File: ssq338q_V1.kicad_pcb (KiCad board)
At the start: 6 copper layers, 32 x 40 mm, 126 parts, among them J4 Conn_01x04_MountingPin, J6 Conn_01x06_MountingPin, J7 Conn_01x03_MountingPin, J8 Conn_01x02_MountingPin, U1 TLV74018PDBVR, U11 W25Q128JVSIQ, U13 BL-M8812EU2, U14 TMI3411, U17 TMI3408F, U2 SSC338Q, U3 MP9943GQ-Z, U7 TMI3113B, X2 24MHz

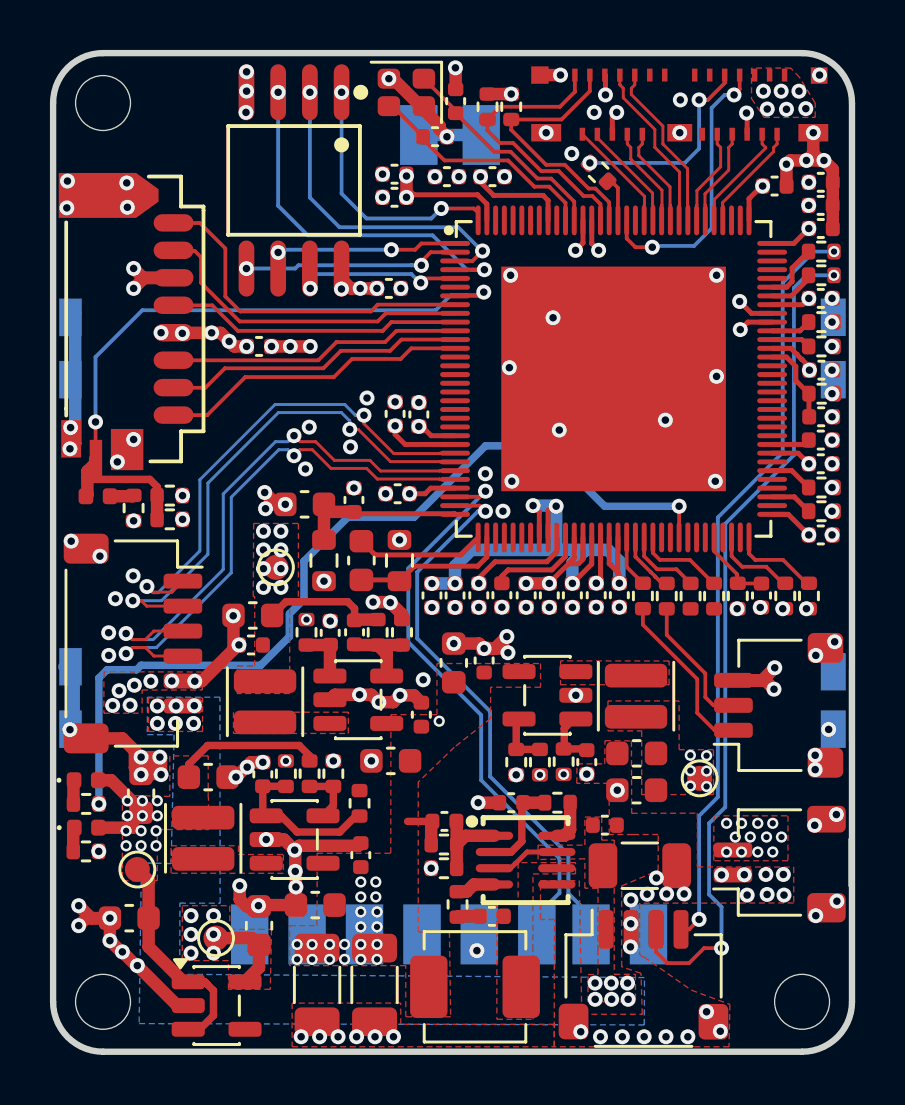
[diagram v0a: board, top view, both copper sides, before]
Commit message: minor changes
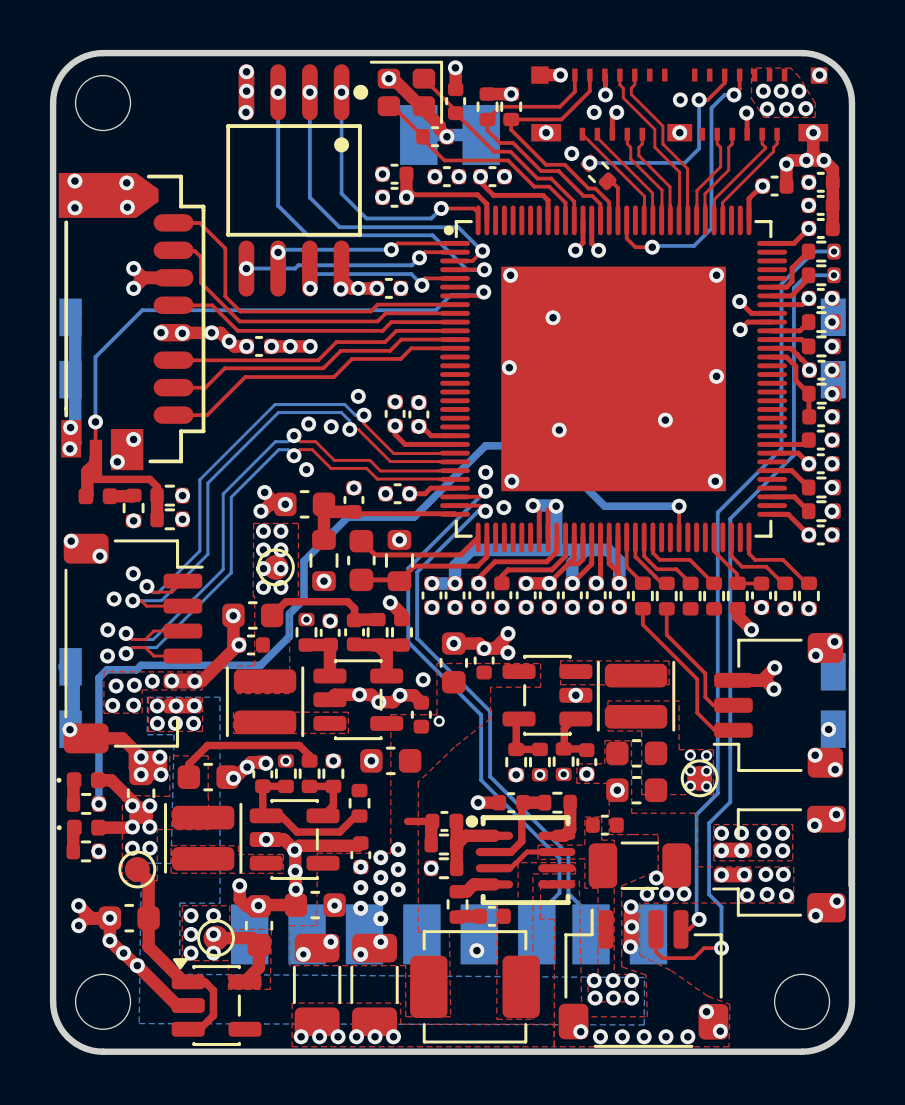
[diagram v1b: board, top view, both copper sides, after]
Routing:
- net +3V3: track 46.4 -> 47.4 mm, vias 43 -> 36
- net GND: track 76.2 -> 76.1 mm, vias 177 -> 176
- net +5V: vias 36 -> 27
